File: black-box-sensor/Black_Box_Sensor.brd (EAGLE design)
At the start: 100 x 80 mm, 34 parts, among them J1 104031-0811, J2 UX60-MB-5S8, J3 B4B-PH-SM4-TBT(LF)(SN), U1 ADXL375, U2 ADXL375, U3 ATMEGA32U4-AU, U4 FXAS21002CQR1, U5 MIC5504-3.3YM5-TR, U6 NL27WZ32USG, U7 MAX7375AXR805T, U8 AD8426ACPZ-WP

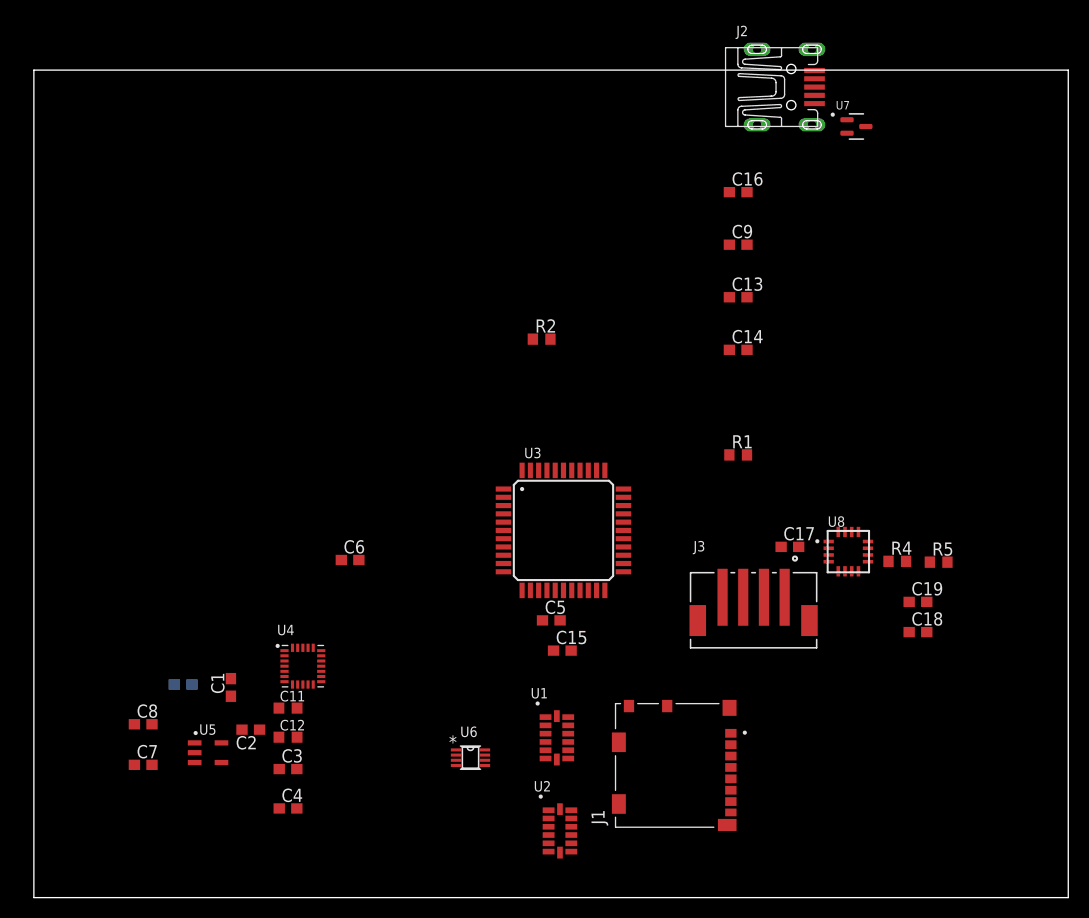
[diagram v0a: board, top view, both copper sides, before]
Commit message: update black box sensor
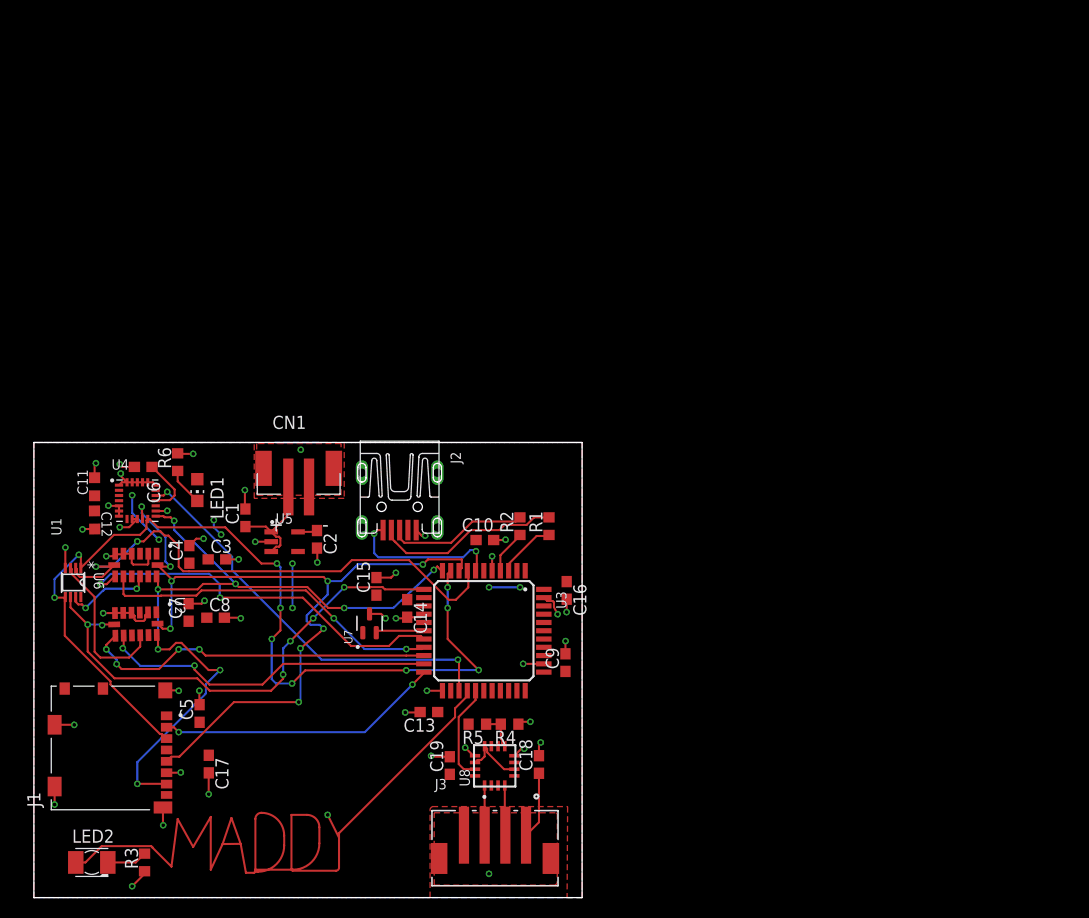
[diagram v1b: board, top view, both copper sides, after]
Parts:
- added CN1: (no value), Hocki_Library:JST-PH-2-SMT
- added LED1: (no value), led:CHIP-LED0805
- added LED2: (no value), led:KA-3528ASYC
- added R3, R6: 100, rcl:R0603
- moved U7 67.2 mm to (32.5, 26.5), turned to 90 degrees
- moved C17 60.0 mm to (16.9, 12.9), turned to 270 degrees
- moved J1 54.6 mm to (7.38, 14.5)
- moved C13 50.0 mm to (38.2, 17.9), turned to 180 degrees
- moved C19 47.9 mm to (40.2, 12.8), turned to 90 degrees
- moved R5 47.3 mm to (42.9, 16.8), turned to 180 degrees
- moved J2 46.5 mm to (35.4, 44.2), turned to 270 degrees
- moved U2 45.6 mm to (9.86, 26.4), turned to 271.1 degrees
- moved U1 44.0 mm to (9.86, 32.1), turned to 270 degrees
- moved C9 43.7 mm to (51.4, 22.7), turned to 90 degrees
- moved U6 42.0 mm to (3.79, 30.5), turned to 270 degrees
- moved C16 41.9 mm to (51.5, 29.7), turned to 270 degrees
- moved R4 40.7 mm to (46.0, 16.8), turned to 180 degrees
- moved C14 40.6 mm to (36.1, 28.0), turned to 270 degrees
- moved U8 40.0 mm to (44.5, 12.7), turned to 90 degrees
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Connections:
- removed net +3.3V: C2.1, U5.5
- removed net ADC9: U3.26, U8.15
- new net CURRENT: U3.27, U8.15
- new net LED: LED2.A, U3.26
- new net N$2: J2.3, R2.2
- new net N$3: J2.4, R1.2
- new net N$5: LED2.C, R3.2
- new net N$6: LED1.C, R6.1
- net 3.3V: now also C2.1, LED1.A, U5.5
- net D+: no longer J2.3, R2.2
- net D-: no longer J2.4, R1.2
- net GND: now also CN1.2, CN1.NC1, CN1.NC2, R3.1, R6.2
- net VBATT: now also CN1.1
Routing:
- net LED: track 0.00 -> 101.2 mm, vias 0 -> 1
- net MOSI: track 0.00 -> 91.9 mm, vias 0 -> 10
- net GND: track 0.00 -> 81.4 mm, vias 0 -> 45
- net SCLK: track 0.00 -> 78.1 mm, vias 0 -> 9
- net MISO: track 0.00 -> 74.5 mm, vias 0 -> 8
- net CS1: track 0.00 -> 51.0 mm, vias 0 -> 2
- net CS2: track 0.00 -> 48.6 mm, vias 0 -> 6
- net CS3: track 0.00 -> 39.9 mm, vias 0 -> 2
- net INT0: track 0.00 -> 37.6 mm, vias 0 -> 2
- net INT2: track 0.00 -> 34.4 mm, vias 0 -> 4
- net INT1: track 0.00 -> 33.5 mm, vias 0 -> 2
- net INT3: track 0.00 -> 32.9 mm, vias 0 -> 2
- net CS4: track 0.00 -> 27.5 mm, vias 0 -> 2
- net 3.3V: track 0.00 -> 22.7 mm, vias 0 -> 8
- net N$3: track 0.00 -> 18.0 mm
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- added copper zone on layer 1, net 3.3V
- added copper zone on layer 1, net GND
- added copper zone on layer 16, net GND
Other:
- board size 100 x 80 mm -> 53 x 44 mm
